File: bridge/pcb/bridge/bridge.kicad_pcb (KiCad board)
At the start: 2 copper layers, 161 x 81 mm, 18 parts, among them J1 Screw_Terminal_01x06, J2 Screw_Terminal_01x06, J3 Screw_Terminal_01x06, J4 Conn_01x23, Q1 PMOS, Q2 PMOS, Q3 PMOS, Q4 PMOS, Q5 PMOS, SW1 SW_SPST, U1 YAAJ_BluePill, U2 J104D2C12VDC.20S

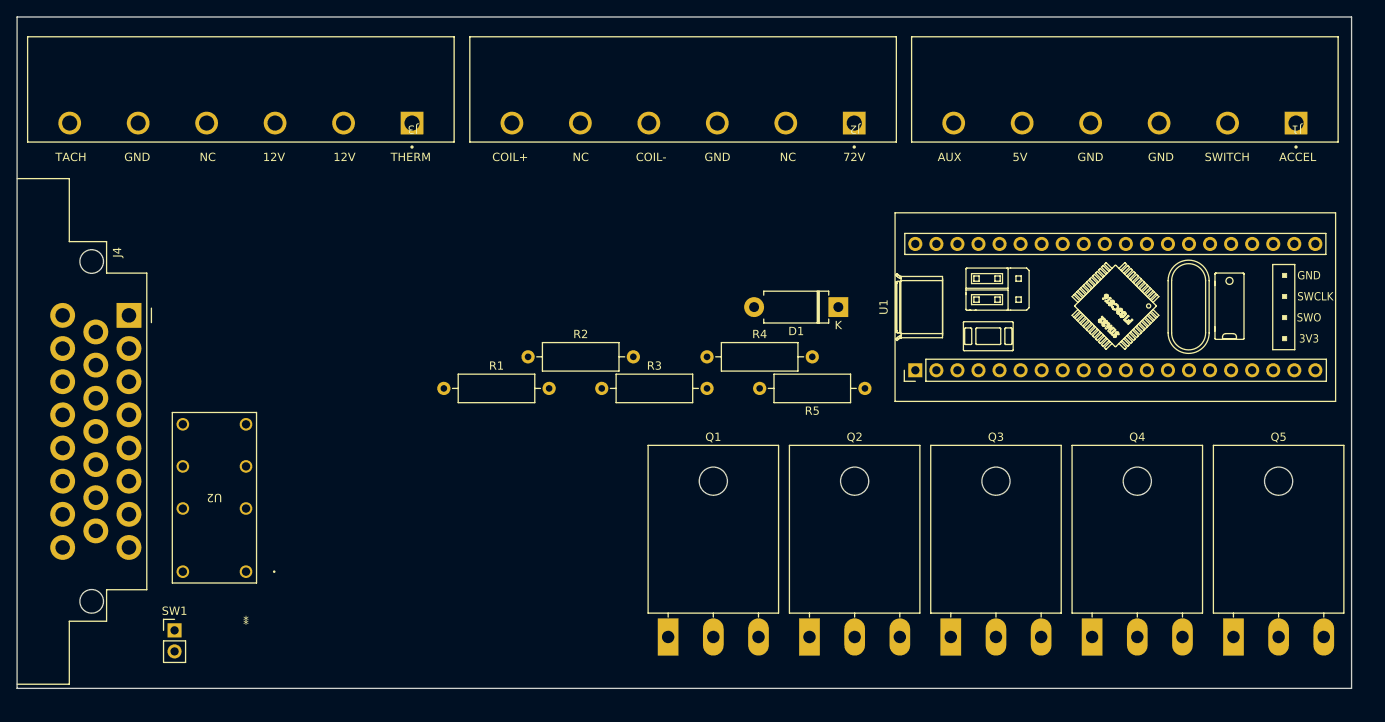
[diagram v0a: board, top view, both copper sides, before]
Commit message: Fixed issues, added DAC
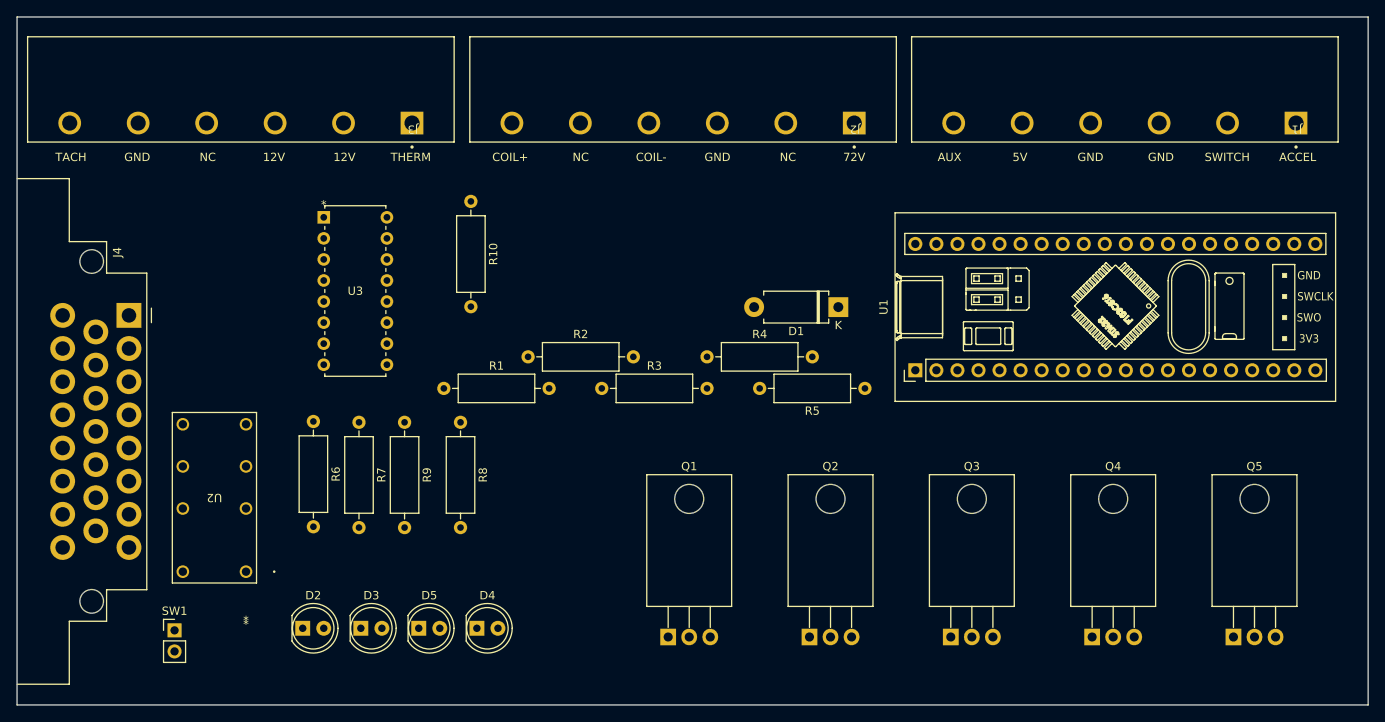
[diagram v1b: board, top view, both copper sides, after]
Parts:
- added D2: GREEN, LED_THT:LED_D5.0mm, F.Cu at (97.5, 114.8)
- added D3: GREEN, LED_THT:LED_D5.0mm, F.Cu at (104.5, 114.8)
- added D4: GREEN, LED_THT:LED_D5.0mm, F.Cu at (118.5, 114.8)
- added D5: GREEN, LED_THT:LED_D5.0mm, F.Cu at (111.5, 114.8)
- added R10: 1k5, Resistor_THT:R_Axial_DIN0309_L9.0mm_D3.2mm_P12.70mm_Horizontal, F.Cu at (117.8, 63.2)
- added R6: 24k, Resistor_THT:R_Axial_DIN0309_L9.0mm_D3.2mm_P12.70mm_Horizontal, F.Cu at (98.8, 89.8)
- added R7: 24k, Resistor_THT:R_Axial_DIN0309_L9.0mm_D3.2mm_P12.70mm_Horizontal, F.Cu at (104.2, 89.9)
- added R8: 10k, Resistor_THT:R_Axial_DIN0309_L9.0mm_D3.2mm_P12.70mm_Horizontal, F.Cu at (116.5, 89.9)
- added R9: 144k, Resistor_THT:R_Axial_DIN0309_L9.0mm_D3.2mm_P12.70mm_Horizontal, F.Cu at (109.8, 89.9)
- added U3: AD557JN, bridge:AD557JN, F.Cu at (100.0, 65.2)
- Q1, Q2, Q3, Q4, Q5: footprint Package_TO_SOT_THT:TO-3P-3_Horizontal_TabDown -> Package_TO_SOT_THT:TO-220-3_Horizontal_TabDown
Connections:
- U1 pad 25: unconnected-(U1-PA0-Pad25) -> Net-(U1-PA0)
- U1 pad 26: unconnected-(U1-PA1-Pad26) -> Net-(U1-PA1)
- U1 pad 27: unconnected-(U1-PA2-Pad27) -> Net-(U1-PA2)
- U1 pad 28: unconnected-(U1-PA3-Pad28) -> Net-(U1-PA3)
- U1 pad 29: unconnected-(U1-PA4-Pad29) -> Net-(U1-PA4)
- U1 pad 30: unconnected-(U1-PA5-Pad30) -> Net-(U1-PA5)
- U1 pad 31: unconnected-(U1-PA6-Pad31) -> Net-(U1-PA6)
- U1 pad 32: unconnected-(U1-PA7-Pad32) -> Net-(U1-PA7)
- U2 pad 4: ACCEL_AUX_AUTO -> unconnected-(U2-Pad4)
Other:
- board size 161 x 81 mm -> 163 x 83 mm
